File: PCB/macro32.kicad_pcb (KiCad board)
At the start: 2 copper layers, 81 x 81 mm, 55 parts, among them J1 USB_C_Receptacle_USB2.0_16P, SW1 RST, SW2 boot, SW3 RotaryEncoder_Switch, SW4 RotaryEncoder_Switch, U1 STM32F072C8Tx, U2 USBLC6-2P6, U3 XC6206PxxxMR, U4 74AHC1G125

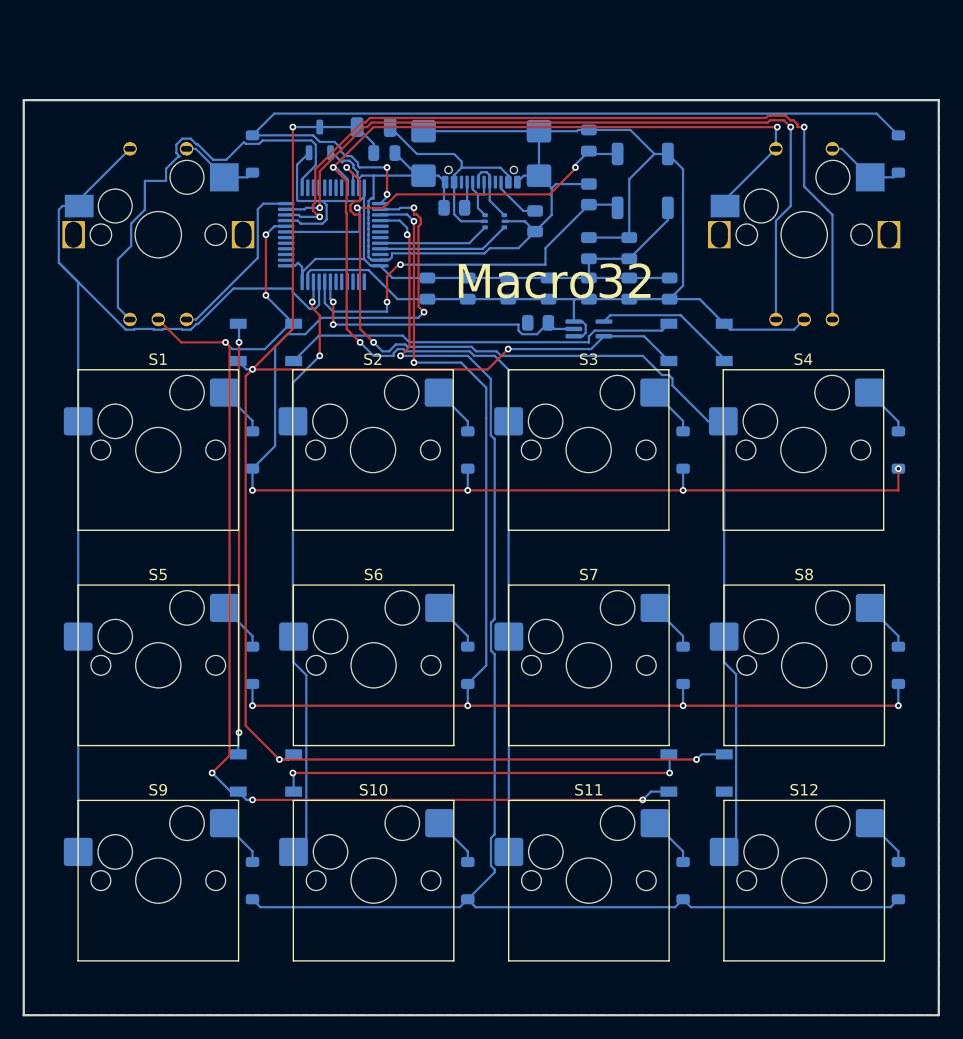
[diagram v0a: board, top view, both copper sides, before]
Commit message: PCB for v2 in the works
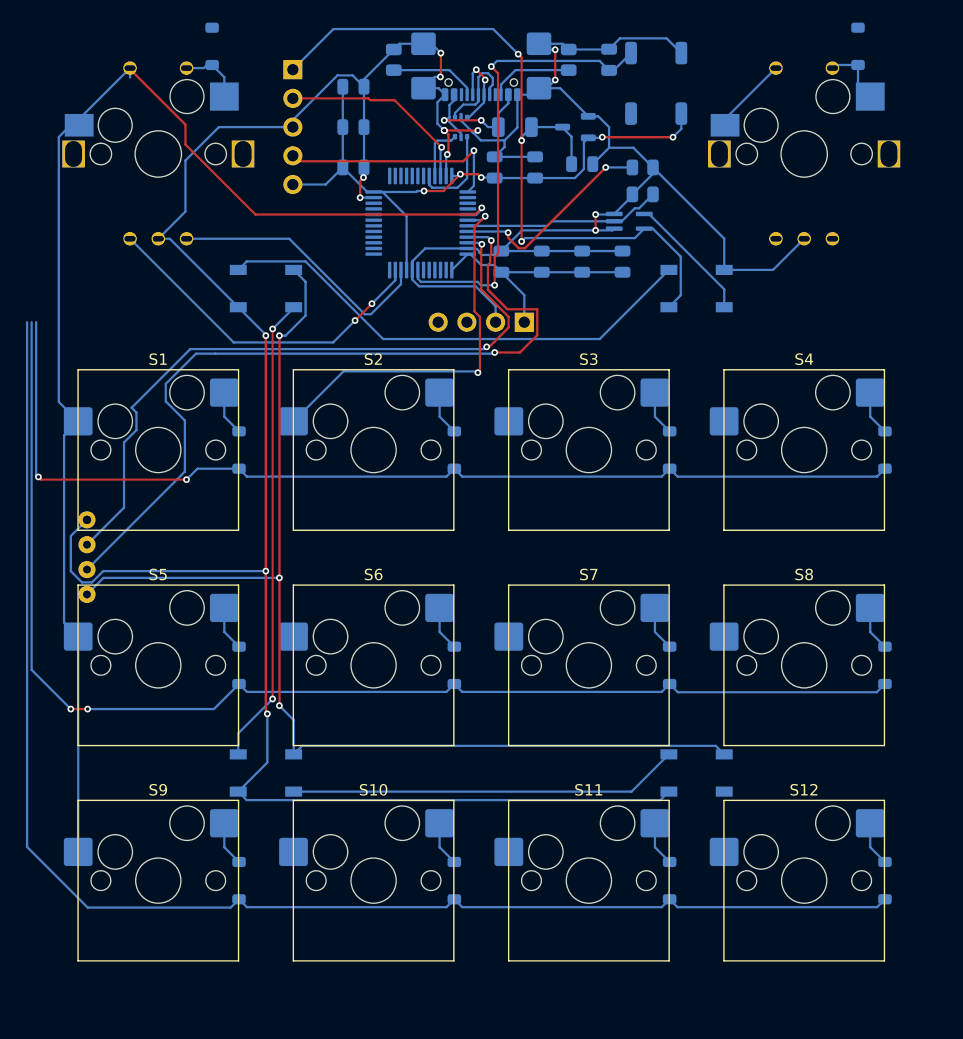
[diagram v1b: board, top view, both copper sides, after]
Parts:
- added J2: Debug header, Connector_PinHeader_2.54mm:PinHeader_1x05_P2.54mm_Vertical, B.Cu at (73.7, 53.7)
- added OL1: OLED, ScottoKeebs_Components:OLED_128x64, F.Cu at (90.4, 76.1)
- added U5: fakeMag4pinFemale, Library:fakemag4pin90degFemale, B.Cu at (55.5, 96.9)
- C1: value 4,7u -> 1u
- C2: value 1u -> 4,7u
- J1: footprint kbd:USB_C_Receptacle_GCT_USB4110 -> Connector_USB:USB_C_Receptacle_GCT_USB4110
- SW2: value boot -> BOOT
- moved C3 31.4 mm to (79.1, 58.8), turned to 0 degrees
- moved C4 28.3 mm to (79.1, 55.3), turned to 0 degrees
- moved C2 26.7 mm to (79.1, 62.4), turned to 0 degrees
- moved U3 22.6 mm to (98.7, 58.8), turned to 180 degrees
- moved C11 17.5 mm to (99.3, 62.1)
- moved R4 14.7 mm to (104.7, 64.8)
- moved R3 14.6 mm to (98.2, 52.9), turned to 90 degrees
- moved R2 14.1 mm to (82.7, 52.9), turned to 90 degrees
- moved C1 13.6 mm to (91.6, 62.4), turned to 90 degrees
- moved F1 12.5 mm to (93.4, 58.8), turned to 0 degrees
- moved C8 10.8 mm to (95.2, 62.4), turned to 90 degrees
- moved C6 10.4 mm to (99.3, 70.7), turned to 90 degrees
- moved C7 10.4 mm to (102.9, 70.7), turned to 90 degrees
- moved D11 10.2 mm to (123.8, 51.7)
- moved D10 10.2 mm to (66.6, 51.7)
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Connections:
- net Net-(U1-BOOT0) renamed BOOT
- net Net-(U1-NRST) renamed RST
- SW3 pad A: encoder2_1 -> encoder1_1
- SW3 pad B: encoder2_0 -> encoder1_0
- SW4 pad A: encoder1_1 -> encoder2_1
- SW4 pad B: encoder1_0 -> encoder2_0
- SW4 pad S2: Col 2 -> Col 3
- U1 pad 14: unconnected-(U1-PA4-Pad14) -> Row 0
- U1 pad 15: unconnected-(U1-PA5-Pad15) -> Row 1
- U1 pad 16: unconnected-(U1-PA6-Pad16) -> Row 2
- U1 pad 17: unconnected-(U1-PA7-Pad17) -> Row 3
- U1 pad 19: unconnected-(U1-PB1-Pad19) -> Col 3
- U1 pad 20: unconnected-(U1-PB2-Pad20) -> Col 2
- U1 pad 21: Col 2 -> SCL_OLED
- U1 pad 22: Col 3 -> SDA_OLED
- U1 pad 25: Row 0 -> unconnected-(U1-PB12-Pad25)
- U1 pad 26: Row 1 -> unconnected-(U1-PB13-Pad26)
- U1 pad 27: Row 2 -> unconnected-(U1-PB14-Pad27)
- U1 pad 28: Row 3 -> unconnected-(U1-PB15-Pad28)
- U1 pad 34: unconnected-(U1-PA13-Pad34) -> SWDIO
- U1 pad 37: unconnected-(U1-PA14-Pad37) -> SWCLK
- U1 pad 41: unconnected-(U1-PB5-Pad41) -> Col 0
- U1 pad 42: unconnected-(U1-PB6-Pad42) -> Col 1
- U1 pad 45: Col 0 -> SCL
- U1 pad 46: Col 1 -> SDA
- U2 pad 3: D+ -> USB D-
- U2 pad 6: USB D- -> D+
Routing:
- net Col 2: track 126.1 -> 0.00 mm, vias 3 -> 0
- net Col 3: track 93.5 -> 6.92 mm, vias 2 -> 0
- net Row 0: track 75.6 -> 0.00 mm, vias 2 -> 0
- net SCL: track 0.00 -> 69.4 mm, vias 0 -> 2
- net SDA: track 0.00 -> 60.1 mm, vias 0 -> 2
- net encoder1_0: track 71.5 -> 24.1 mm, vias 2 -> 0
- net encoder2_1: track 38.1 -> 0.00 mm
- net encoder1_1: track 67.6 -> 30.5 mm
- net GND: track 268.4 -> 305.1 mm, vias 6 -> 15
- net SWCLK: track 0.00 -> 20.5 mm, vias 0 -> 1
- net +5V: track 149.7 -> 168.9 mm, vias 5 -> 6
- net Col 1: track 52.7 -> 34.4 mm
- net Col 0: track 96.6 -> 114.4 mm, vias 0 -> 1
- net SWDIO: track 0.00 -> 17.5 mm, vias 0 -> 1
- net BOOT: track 34.8 -> 18.4 mm
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- removed copper zone on B.Cu, net GND
- removed copper zone on F.Cu, net GND
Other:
- board outline removed
- board text removed: "Macro32"
